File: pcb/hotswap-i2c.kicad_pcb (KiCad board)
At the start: 2 copper layers, 17.2 x 11.2 mm, 7 parts, among them J1 Conn_01x04_Male, J2 Conn_01x04_Male, U1 TCA4311ADR

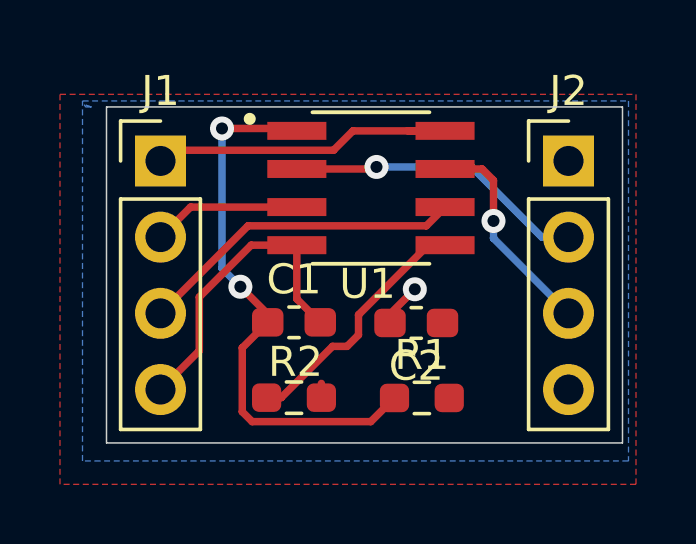
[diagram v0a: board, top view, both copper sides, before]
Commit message: some rerouting
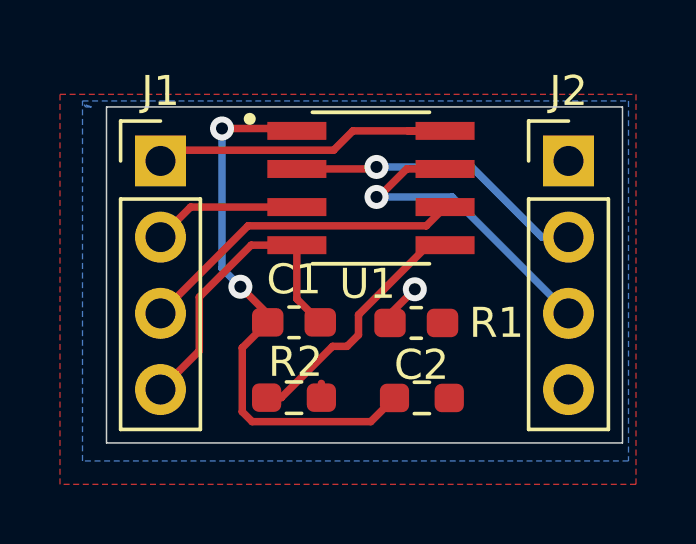
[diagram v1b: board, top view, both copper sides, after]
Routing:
- net SDAOUT: track 7.24 -> 10.7 mm
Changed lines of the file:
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@@
     (tags "capacitor handsolder")
     (attr smd)
-    (fp_text reference C2 (at 0 -1.43) (layer F.SilkS)
+    (fp_text reference C2 (at -0.175 -1.4) (layer F.SilkS)
       (effects (font (size 1 1) (thickness 0.15)))
     )
     (fp_text value 0.01uF (at 0 1.43) (layer F.Fab)
       (effects (font (size 1 1) (thickness 0.15)))
-    )
-    (fp_text user %R (at 0 0) (layer F.Fab)
-      (effects (font (size 0.4 0.4) (thickness 0.06)))
     )
     (fp_line (start -0.8 0.4) (end -0.8 -0.4) (layer F.Fab) (width 0.1))
@@
     (fp_line (start 1.65 -0.73) (end 1.65 0.73) (layer F.CrtYd) (width 0.05))
     (fp_line (start 1.65 0.73) (end -1.65 0.73) (layer F.CrtYd) (width 0.05))
+    (fp_text user %R (at 0 0) (layer F.Fab)
+      (effects (font (size 0.4 0.4) (thickness 0.06)))
+    )
     (pad 2 smd roundrect (at 0.875 0 180) (size 1.05 0.95) (layers F.Cu F.Paste F.Mask) (roundrect_rratio 0.25)
       (net 1 GND))
@@
     (tags "resistor handsolder")
     (attr smd)
-    (fp_text reference R1 (at 0 -1.43) (layer F.SilkS)
+    (fp_text reference R1 (at 2.4875 -2.5) (layer F.SilkS)
       (effects (font (size 1 1) (thickness 0.15)))
     )
@@
   (segment (start 142.2525 80.3575) (end 145.795 80.3575) (width 0.25) (layer F.Cu) (net 3))
   (segment (start 141.25 81.36) (end 142.2525 80.3575) (width 0.25) (layer F.Cu) (net 3))
-  (via (at 152.35 80.82) (size 0.8) (drill 0.4) (layers F.Cu B.Cu) (net 4))
-  (segment (start 152.35 79.4675) (end 152.35 80.82) (width 0.25) (layer F.Cu) (net 4))
-  (segment (start 151.97 79.0875) (end 152.35 79.4675) (width 0.25) (layer F.Cu) (net 4))
-  (segment (start 150.735 79.0875) (end 151.97 79.0875) (width 0.25) (layer F.Cu) (net 4))
-  (segment (start 152.35 81.4) (end 154.85 83.9) (width 0.25) (layer B.Cu) (net 4))
-  (segment (start 152.35 80.82) (end 152.35 81.4) (width 0.25) (layer B.Cu) (net 4))
+  (via (at 148.45 80.020003) (size 0.8) (drill 0.4) (layers F.Cu B.Cu) (net 4))
+  (segment (start 148.522999 80.020003) (end 148.45 80.020003) (width 0.25) (layer F.Cu) (net 4))
+  (segment (start 149.455502 79.0875) (end 148.522999 80.020003) (width 0.25) (layer F.Cu) (net 4))
+  (segment (start 150.735 79.0875) (end 149.455502 79.0875) (width 0.25) (layer F.Cu) (net 4))
+  (segment (start 150.970003 80.020003) (end 154.85 83.9) (width 0.25) (layer B.Cu) (net 4))
+  (segment (start 148.45 80.020003) (end 150.970003 80.020003) (width 0.25) (layer B.Cu) (net 4))
   (via (at 148.45 79.02) (size 0.8) (drill 0.4) (layers F.Cu B.Cu) (net 5))
   (segment (start 148.3825 79.0875) (end 148.45 79.02) (width 0.25) (layer F.Cu) (net 5))
